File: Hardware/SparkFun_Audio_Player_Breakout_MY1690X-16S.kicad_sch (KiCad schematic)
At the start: 40 parts, among them J1 3.5mm TRRS, J2 Conn_01x03, J3 Conn_01x02, J4 USB_C_Receptacle, J5 Conn_01x06, J6 microSD, Q1 BSS138, U2 MY1690X-16S

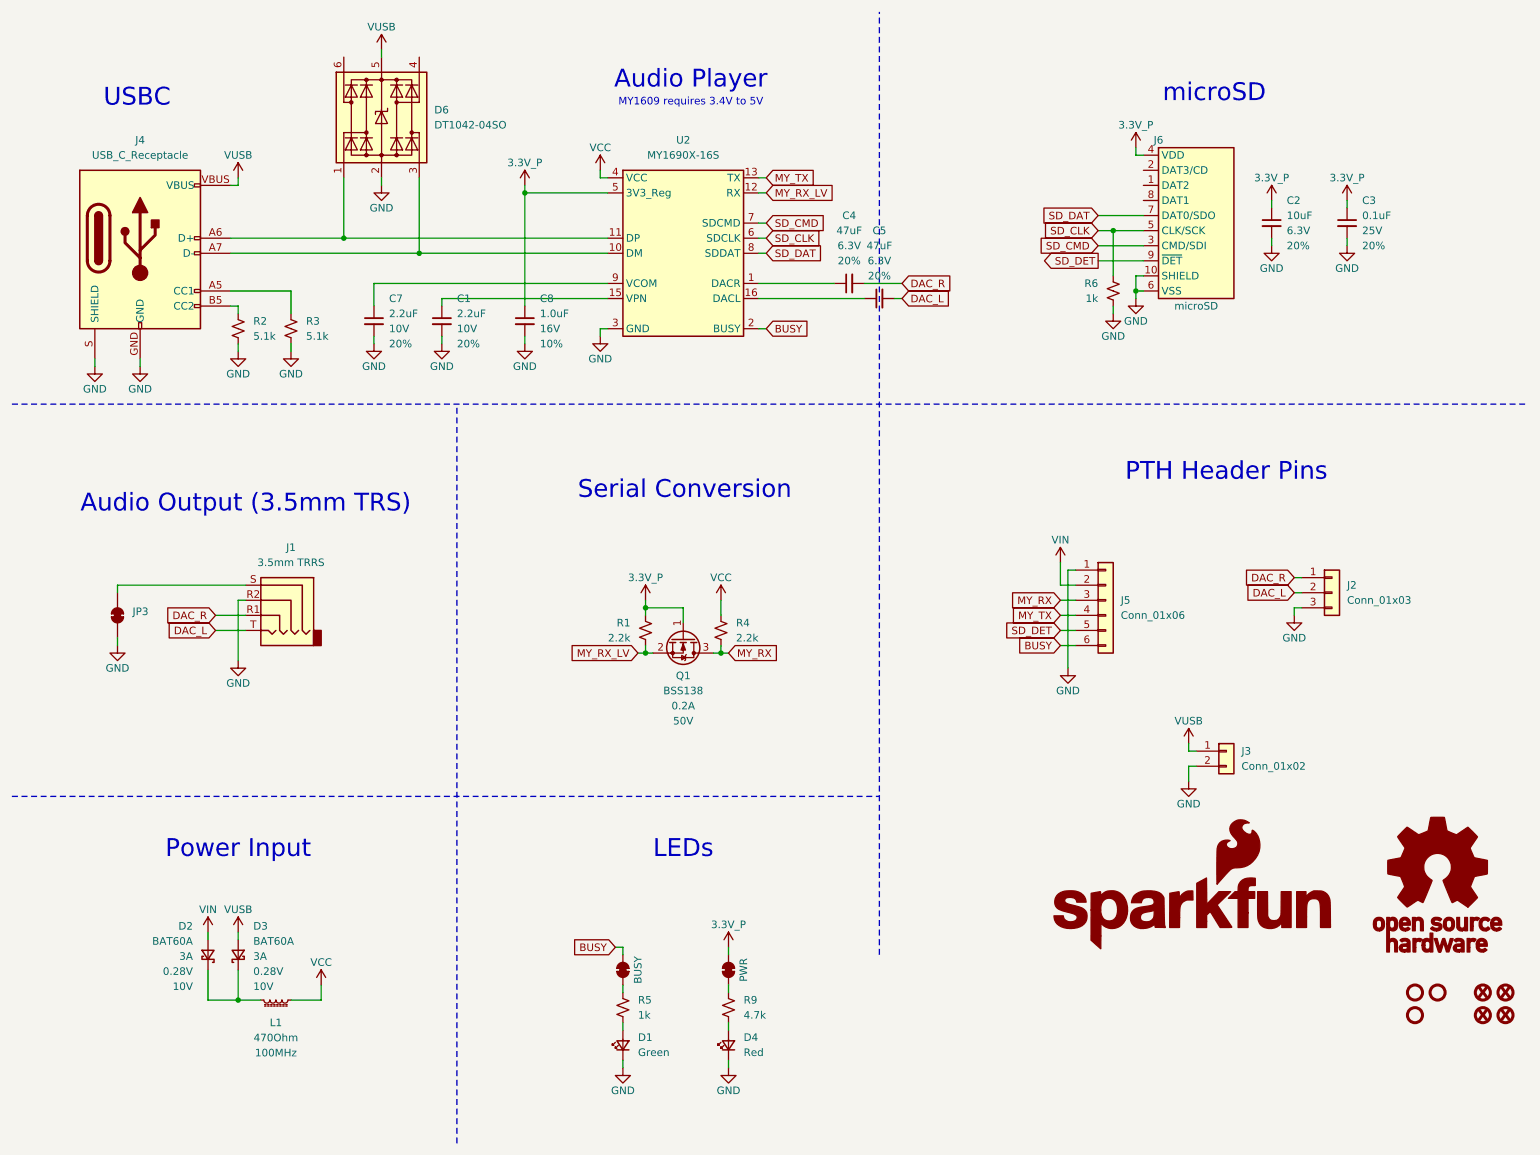
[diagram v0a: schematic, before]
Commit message: Routed v01 (pre-review)
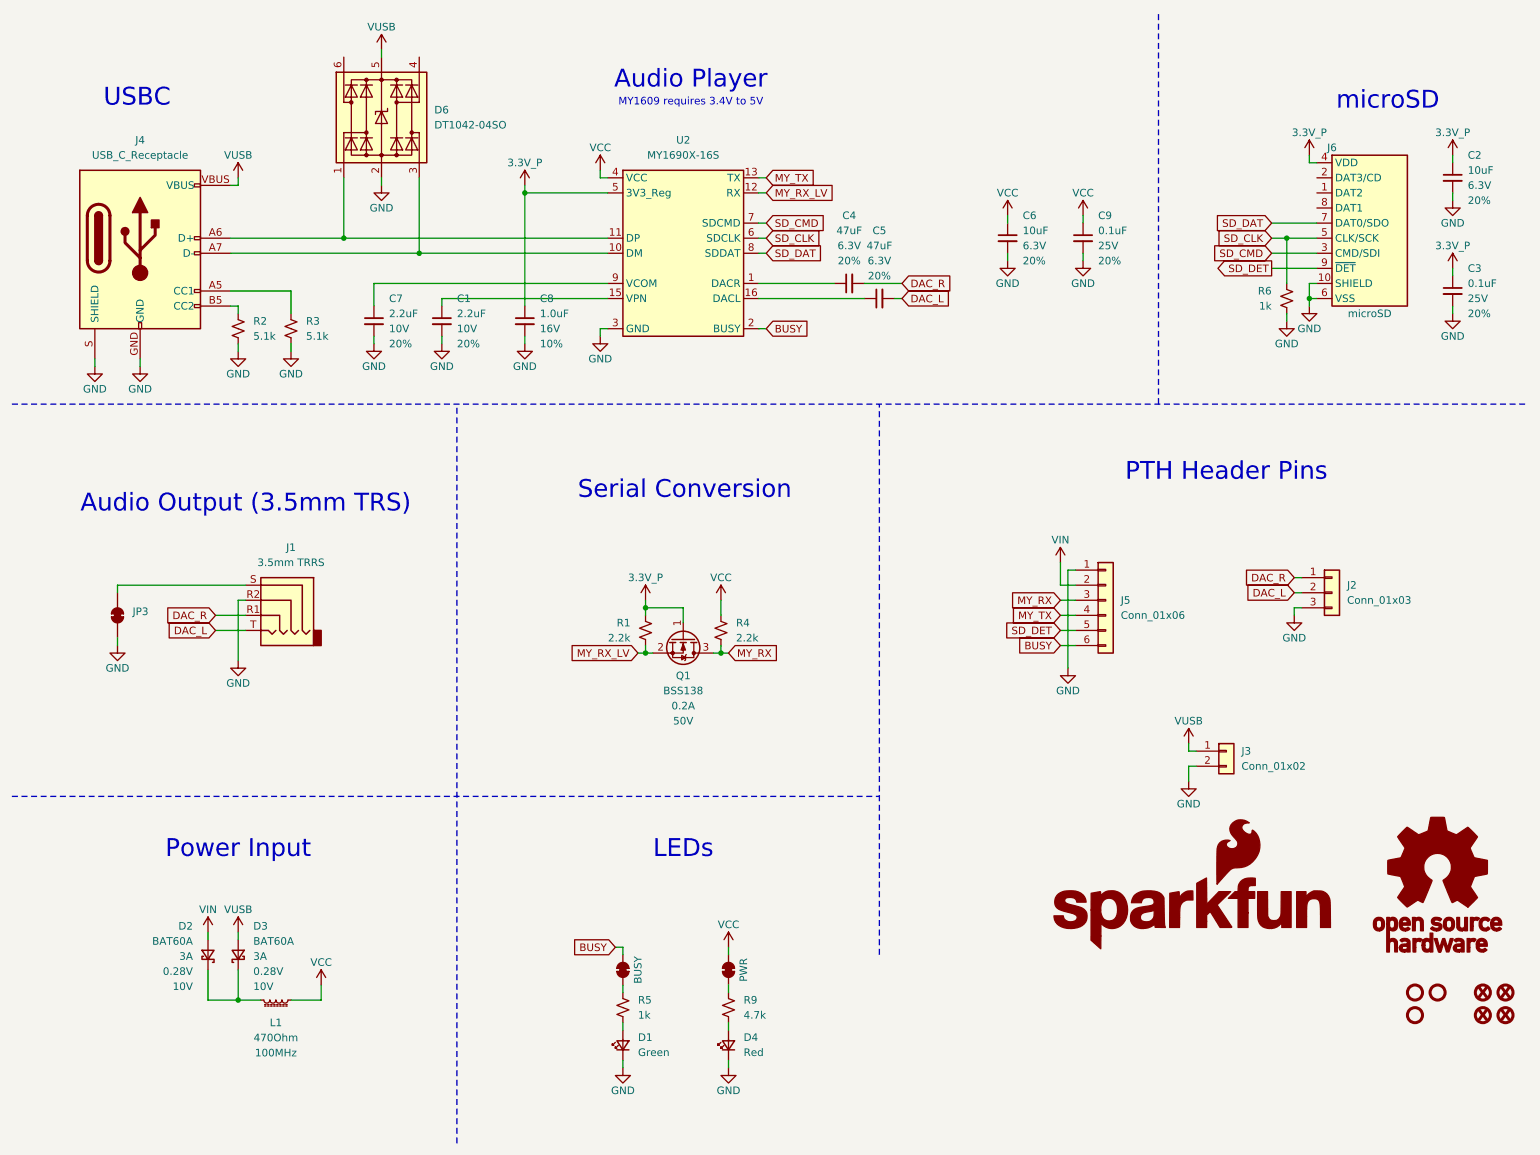
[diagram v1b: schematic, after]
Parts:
- added C6: 10uF, SparkFun-Capacitor:C_0603_1608Metric, symbol SparkFun-Capacitor:10uF_0603_6.3V_20%
- added C9: 0.1uF, SparkFun-Capacitor:C_0603_1608Metric, symbol SparkFun-Capacitor:0.1uF_0603_25V_20%
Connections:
- net 3.3V_P: no longer JP2.2 (B)
- net GND: now also C6.2, C9.2
- net VCC: now also JP2.2 (B), C6.1, C9.1
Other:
- moved on the sheet: C2, C3, J6, R6
